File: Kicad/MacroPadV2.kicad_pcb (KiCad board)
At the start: 2 copper layers, 88.5 x 82.2 mm, 31 parts, among them K1 KSW, K10 KSW, K11 KSW, K12 KSW, K2 KSW, K3 KSW, K4 KSW, K5 KSW, K6 KSW, K7 KSW, K8 KSW, K9 KSW, SW1 RotaryEncoder_Switch, U1 SparkFunProMicro

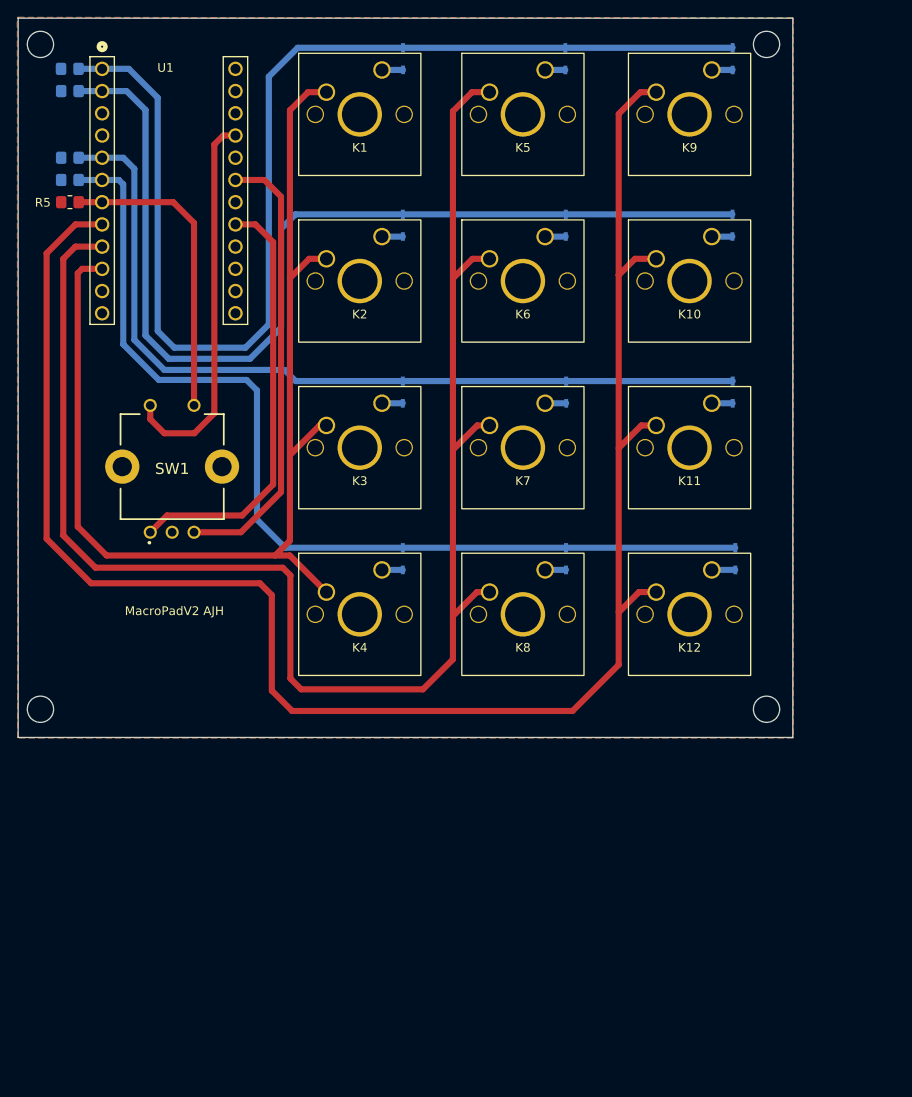
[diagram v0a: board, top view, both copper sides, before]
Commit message: New LAyout an Routing done
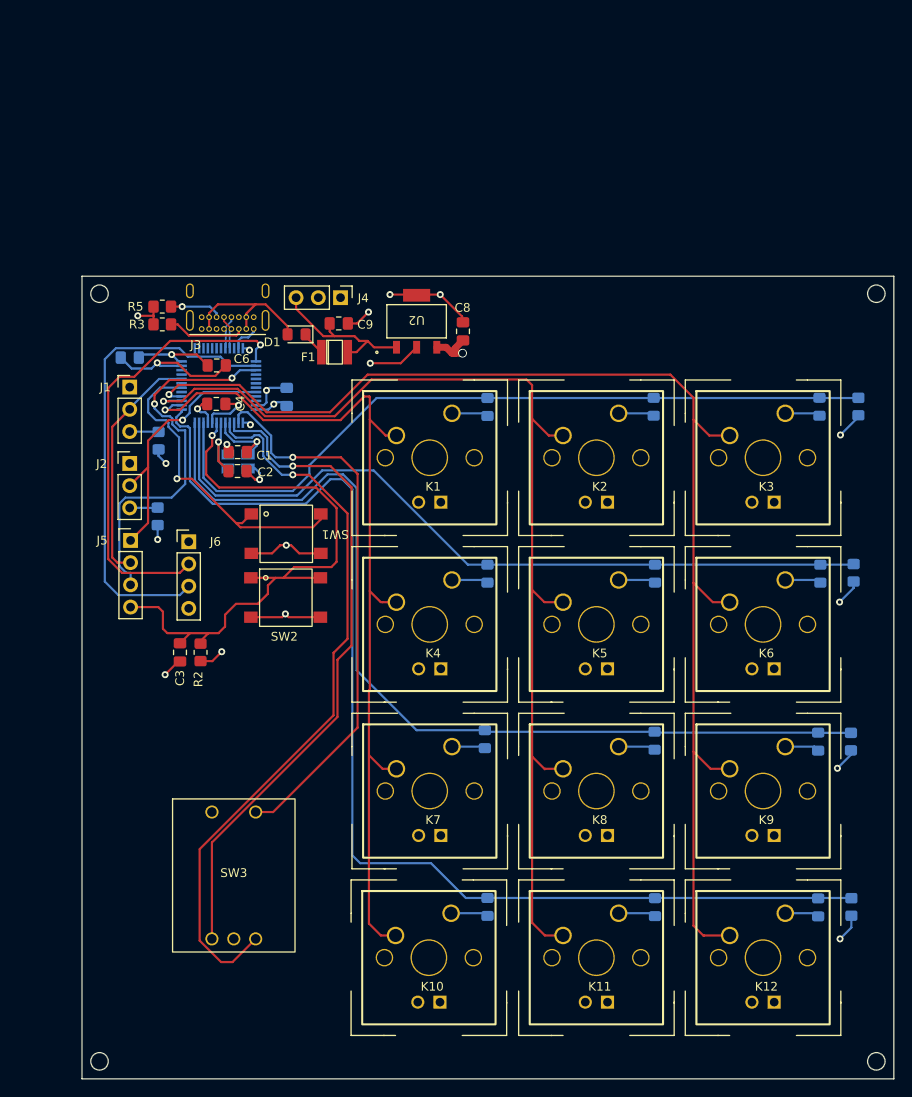
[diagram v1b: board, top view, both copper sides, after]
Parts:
- added C1: 15pF, Capacitor_SMD:C_0805_2012Metric_Pad1.18x1.45mm_HandSolder, F.Cu at (58.5, 70.6)
- added C2: 15pF, Capacitor_SMD:C_0805_2012Metric_Pad1.18x1.45mm_HandSolder, F.Cu at (58.5, 72.8)
- added C3: 100nF, Capacitor_SMD:C_0805_2012Metric_Pad1.18x1.45mm_HandSolder, F.Cu at (52.0, 93.5)
- added C4: 100nF, Capacitor_SMD:C_0805_2012Metric_Pad1.18x1.45mm_HandSolder, F.Cu at (56.1, 65.1)
- added C5: 100nF, Capacitor_SMD:C_0805_2012Metric_Pad1.18x1.45mm_HandSolder, B.Cu at (46.2, 59.8)
- added C6: 1uF, Capacitor_SMD:C_0805_2012Metric_Pad1.18x1.45mm_HandSolder, F.Cu at (56.1, 60.7)
- added C7: 4.7uF, Capacitor_SMD:C_0805_2012Metric_Pad1.18x1.45mm_HandSolder, B.Cu at (64.2, 64.3)
- added C8: 4.7uF, Capacitor_SMD:C_0805_2012Metric_Pad1.18x1.45mm_HandSolder, F.Cu at (84.3, 56.8)
- added C9: 4.7uF, Capacitor_SMD:C_0805_2012Metric_Pad1.18x1.45mm_HandSolder, F.Cu at (70.1, 55.9)
- added D13: 1N4148WX-TP, Diode_SMD:D_0805_2012Metric_Pad1.15x1.40mm_HandSolder, B.Cu at (125.0, 65.4)
- added F1: OZCH, mpadfps:OZCHFusr, F.Cu at (68.1, 59.2)
- added J1: 3PinJump, Connector_PinHeader_2.54mm:PinHeader_1x03_P2.54mm_Vertical, F.Cu at (46.2, 63.2)
- added J2: 3PinJump, Connector_PinHeader_2.54mm:PinHeader_1x03_P2.54mm_Vertical, F.Cu at (46.2, 71.9)
- added J3: GCT-USB4085, mpadfps:USB4085-GF-A, F.Cu at (57.4, 56.5)
- added J4: 3PinJump, Connector_PinHeader_2.54mm:PinHeader_1x03_P2.54mm_Vertical, F.Cu at (70.3, 53.0)
- added J5: 4PinJump, Connector_PinHeader_2.54mm:PinHeader_1x04_P2.54mm_Vertical, F.Cu at (46.3, 80.7)
- added J6: 4PinJump, Connector_PinHeader_2.54mm:PinHeader_1x04_P2.54mm_Vertical, F.Cu at (53.0, 80.8)
- added R6: 1k, Resistor_SMD:R_0805_2012Metric_Pad1.20x1.40mm_HandSolder, B.Cu at (128.7, 122.6)
- added R7: 1k, Resistor_SMD:R_0805_2012Metric_Pad1.20x1.40mm_HandSolder, B.Cu at (128.7, 103.7)
- added R8: 1k, Resistor_SMD:R_0805_2012Metric_Pad1.20x1.40mm_HandSolder, B.Cu at (128.9, 84.4)
- added R9: 1k, Resistor_SMD:R_0805_2012Metric_Pad1.20x1.40mm_HandSolder, B.Cu at (129.5, 65.4)
- added SW2: SWITCH_TACTILE_SPST-NO_0.05A_12V, mpadfps:PTS645-G, F.Cu at (60.0, 85.0)
- added SW3: RotaryEncoder_Switch, mpadfps:PEC11H-RotaryEncoderSwitch, F.Cu at (58.1, 118.8)
- added U2: AP2114HA-3.3TRG1, keyboard_fp:SOT-223_DIO-L, F.Cu at (79.0, 55.6)
- added X1: TSX-3225_16.0000MF18X-AC6, mpadfps:TSX-3226, B.Cu at (58.5, 71.6)
- D1: value KD -> D; footprint mpadfps:sod323 -> Diode_SMD:D_0805_2012Metric_Pad1.15x1.40mm_HandSolder; moved to F.Cu
- D10, D11, D12, D2, D3, D4, D5, D6, D7, D8, D9: value KD -> 1N4148WX-TP; footprint mpadfps:sod323 -> Diode_SMD:D_0805_2012Metric_Pad1.15x1.40mm_HandSolder
- K1, K10, K11, K12, K2, K3, K4, K5, K6, K7, K8, K9: footprint aarohanl:CherryMxFP -> keyboard_fp:CherryMx
- R1, R4: value 1k -> 10k
- R2: value 1k -> 10k; moved to F.Cu
- R3: value 1k -> 5.1k; moved to F.Cu
- R5: value 1k -> 5.1k
- SW1: value RotaryEncoder_Switch -> SWITCH_TACTILE_SPST-NO_0.05A_12V; footprint aarohanl:PEC11H4020FS0016_PinCorrection -> mpadfps:PTS645-G
- U1: value SparkFunProMicro -> STM32F103C8T6TR; footprint aarohanl:SparkFrunProMicro -> mpadfps:LQFP48; moved to B.Cu
- moved D9 98.4 mm to (106.2, 122.6), turned to 90 degrees
- moved K10 82.9 mm to (80.4, 128.4)
- moved K9 77.8 mm to (118.6, 109.3)
- moved R2 65.9 mm to (54.3, 93.5), turned to 90 degrees
- moved K11 59.3 mm to (99.5, 128.4)
- moved K5 58.9 mm to (99.5, 90.3)
- moved K6 47.9 mm to (118.6, 90.3)
- moved K3 46.1 mm to (118.6, 71.2)
- moved R1 43.7 mm to (49.5, 69.3), turned to -90 degrees
- moved D11 42.1 mm to (124.9, 103.7), turned to 90 degrees
- moved D10 42.1 mm to (125.2, 84.5), turned to 90 degrees
- moved D2 42.0 mm to (87.1, 84.5), turned to 90 degrees
- moved D12 42.0 mm to (124.9, 122.7), turned to 90 degrees
- moved D4 42.0 mm to (87.1, 122.6), turned to 90 degrees
- moved D5 41.8 mm to (87.1, 65.5), turned to 90 degrees
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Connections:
- D1 pad 1: COL0 -> Net-(D1-Pad1)
- D1 pad 2: Net-(D1-Pad2) -> VBUS
- D10 pad 1: COL1 -> Net-(D10-Pad1)
- D10 pad 2: Net-(D10-Pad2) -> ROW1
- D11 pad 1: COL2 -> Net-(D11-Pad1)
- D11 pad 2: Net-(D11-Pad2) -> ROW2
- D12 pad 1: COL3 -> Net-(D12-Pad1)
- D12 pad 2: Net-(D12-Pad2) -> ROW3
- D2 pad 1: COL1 -> Net-(D2-Pad1)
- D2 pad 2: Net-(D2-Pad2) -> ROW1
- D3 pad 1: COL2 -> Net-(D3-Pad1)
- D3 pad 2: Net-(D3-Pad2) -> ROW2
- D4 pad 1: COL3 -> Net-(D4-Pad1)
- D4 pad 2: Net-(D4-Pad2) -> ROW3
- D5 pad 1: COL0 -> Net-(D5-Pad1)
- D5 pad 2: Net-(D5-Pad2) -> ROW0
- D6 pad 1: COL1 -> Net-(D6-Pad1)
- D6 pad 2: Net-(D6-Pad2) -> ROW0
- D7 pad 1: COL2 -> Net-(D7-Pad1)
- D7 pad 2: Net-(D7-Pad2) -> ROW1
- D8 pad 1: COL3 -> Net-(D8-Pad1)
- D8 pad 2: Net-(D8-Pad2) -> ROW2
- D9 pad 1: COL0 -> Net-(D9-Pad1)
- D9 pad 2: Net-(D9-Pad2) -> ROW3
- K1 pad 1: ROW0 -> COL0
- K1 pad 2: Net-(D1-Pad2) -> Net-(D5-Pad1)
- K10 pad 1: ROW2 -> COL0
- K10 pad 2: Net-(D10-Pad2) -> Net-(D4-Pad1)
- K11 pad 1: ROW2 -> COL1
- K11 pad 2: Net-(D11-Pad2) -> Net-(D9-Pad1)
- K12 pad 1: ROW2 -> COL2
- K12 pad 2: Net-(D12-Pad2) -> Net-(D12-Pad1)
- K2 pad 1: ROW0 -> COL1
- K2 pad 2: Net-(D2-Pad2) -> Net-(D6-Pad1)
- K3 pad 1: ROW0 -> COL2
- K3 pad 2: Net-(D3-Pad2) -> Net-(D13-Pad1)
- K4 pad 1: ROW0 -> COL0
- K4 pad 2: Net-(D4-Pad2) -> Net-(D2-Pad1)
- K5 pad 1: ROW1 -> COL1
- K5 pad 2: Net-(D5-Pad2) -> Net-(D7-Pad1)
- K6 pad 1: ROW1 -> COL2
- K6 pad 2: Net-(D6-Pad2) -> Net-(D10-Pad1)
- K7 pad 1: ROW1 -> COL0
- K7 pad 2: Net-(D7-Pad2) -> Net-(D3-Pad1)
- K8 pad 1: ROW1 -> COL1
- K8 pad 2: Net-(D8-Pad2) -> Net-(D8-Pad1)
- K9 pad 1: ROW2 -> COL2
- K9 pad 2: Net-(D9-Pad2) -> Net-(D11-Pad1)
- R1 pad 1: COL0 -> Net-(J1-Pad3)
- R2 pad 1: COL1 -> +3V3
- R2 pad 2: GND -> NRST
- R3 pad 1: COL2 -> GND
- R3 pad 2: GND -> Net-(J3-PadA5)
- R4 pad 1: COL3 -> Net-(J2-Pad3)
- R5 pad 1: PD4 -> GND
- R5 pad 2: GND -> Net-(J3-PadB5)
- U1 pad 1: COL0 -> +3V3
- U1 pad 11: PB4 -> ROW1
- U1 pad 12: PB5 -> ROW2
- U1 pad 13: unconnected-(U1-Pad13) -> ROW3
- U1 pad 14: GND -> COL0
- U1 pad 15: unconnected-(U1-Pad15) -> COL1
- U1 pad 16: VCC -> COL2
- U1 pad 17: PF4 -> unconnected-(U1-Pad17)
- U1 pad 18: PF6 -> MODE
- U1 pad 19: (no net) -> unconnected-(U1-Pad19)
- U1 pad 2: COL1 -> ENCSW
- U1 pad 20: PF7 -> BOOT1
- U1 pad 21: PB1 -> unconnected-(U1-Pad21)
- U1 pad 22: PB3 -> unconnected-(U1-Pad22)
- U1 pad 23: PB2 -> GND
- U1 pad 24: PB6 -> +3V3
- U1 pad 3: GND -> ENCA
- U1 pad 4: GND -> ENCB
- U1 pad 5: COL2 -> Net-(C1-Pad2)
- U1 pad 6: COL3 -> Net-(C2-Pad1)
- U1 pad 7: PD4 -> NRST
- U1 pad 8: ROW2 -> GND
- U1 pad 9: ROW1 -> +3V3
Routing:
- net ROW3: track 0.00 -> 131.8 mm
- net COL3: track 111.8 -> 0.00 mm
- net ROW2: track 206.5 -> 108.2 mm
- net GND: track 0.00 -> 95.6 mm, vias 0 -> 19
- net ROW1: track 180.3 -> 87.7 mm
- net ENCB: track 0.00 -> 84.1 mm, vias 0 -> 1
- net ENCA: track 0.00 -> 76.4 mm, vias 0 -> 1
- net NRST: track 0.00 -> 70.0 mm, vias 0 -> 1
- net ENCSW: track 0.00 -> 63.4 mm, vias 0 -> 1
- net SWCLK: track 0.00 -> 54.7 mm
- net SWDIO: track 0.00 -> 51.8 mm, vias 0 -> 1
- net PF6: track 51.6 -> 0.00 mm
- net COL2: track 96.7 -> 146.0 mm, vias 0 -> 1
- net PF7: track 49.2 -> 0.00 mm
- net VCC: track 44.1 -> 0.00 mm
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- added copper zone on In1.Cu, net +3V3
- added copper zone on In2.Cu, net GND
- removed copper zone on B.Cu, net GND
- removed copper zone on F.Cu, net GND
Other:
- board size 88.5 x 82.2 mm -> 92.8 x 91.8 mm
- copper layers 2 -> 4
- board text removed: "MacroPadV2 AJH"
